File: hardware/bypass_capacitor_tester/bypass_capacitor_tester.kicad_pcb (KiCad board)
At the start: 2 copper layers, 17 x 28.8 mm, 13 parts, among them J1 Coax, J2 Coax, J3 Coax, J4 Conn_01x02, Q1 MMBT2369AL

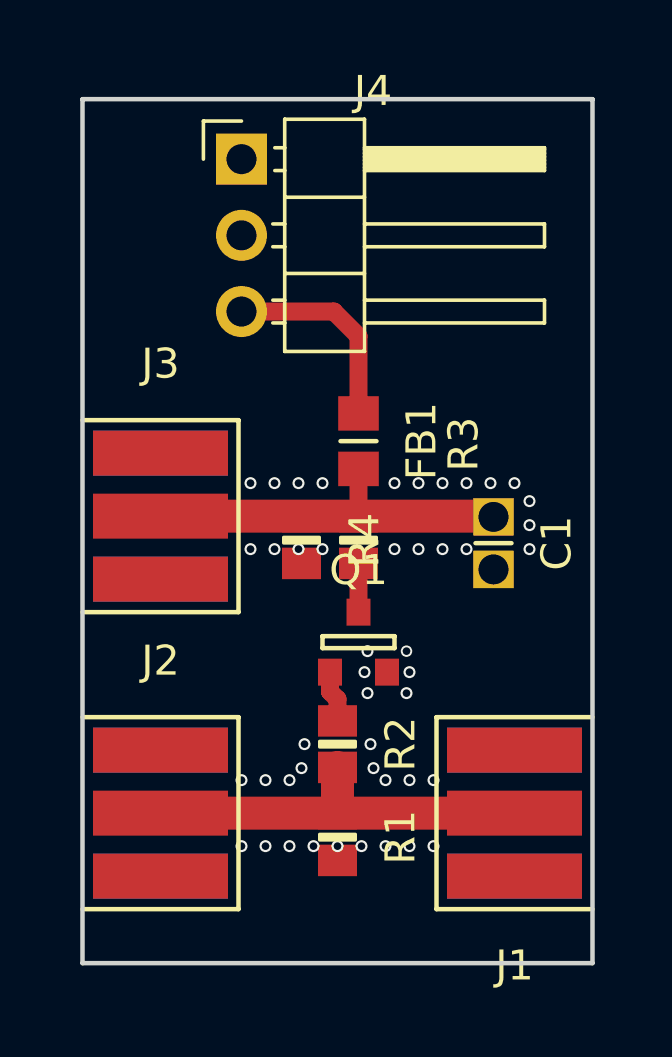
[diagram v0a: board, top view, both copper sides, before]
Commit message: silk placement completed
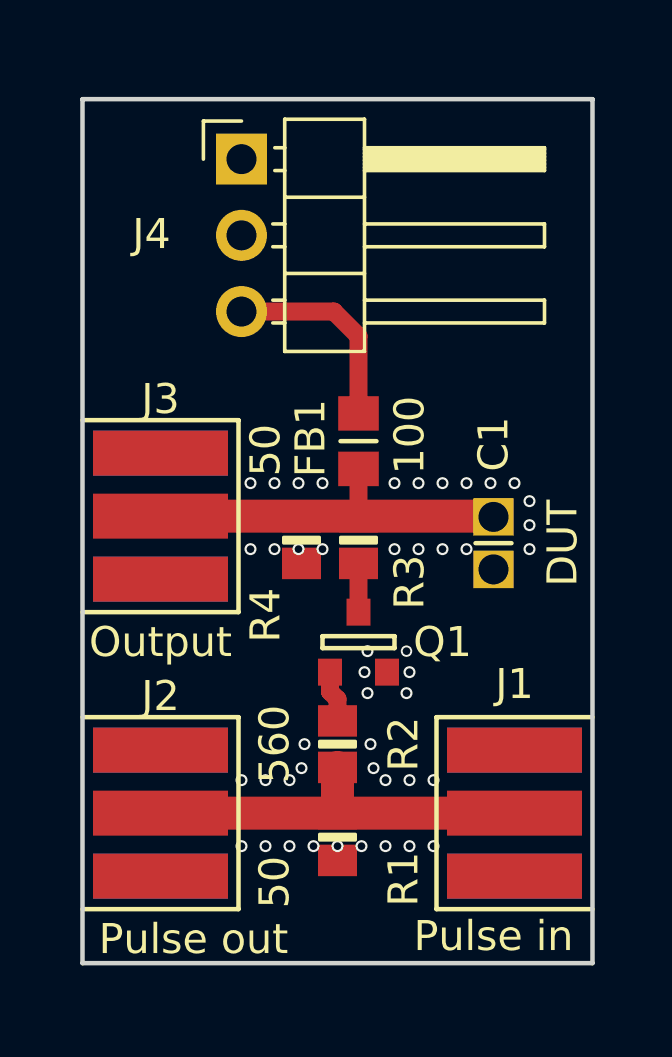
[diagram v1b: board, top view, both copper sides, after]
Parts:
- J1: value Coax -> Pulse in
- J2: value Coax -> Pulse out
- J3: value Coax -> Output
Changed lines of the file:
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@@
     (tags "capacitor 0805 0603 0402 Through hole mixed")
     (attr smd)
-    (fp_text reference C1 (at 0 -2.1 90) (layer F.SilkS)
-      (effects (font (size 1 1) (thickness 0.15)))
-    )
-    (fp_text value DUT (at 0 2.1 90) (layer F.Fab)
+    (fp_text reference C1 (at -3.3 0 90) (layer F.SilkS)
+      (effects (font (size 1 1) (thickness 0.15)))
+    )
+    (fp_text value DUT (at 0 -2.3 90) (layer F.SilkS)
       (effects (font (size 1 1) (thickness 0.15)))
     )
@@
     (descr "Through hole angled pin header, 1x03, 2.54mm pitch, 6mm pin length, single row")
     (tags "Through hole angled pin header THT 1x03 2.54mm single row")
-    (fp_text reference J4 (at 4.385 -2.27) (layer F.SilkS)
+    (fp_text reference J4 (at -3 2.5) (layer F.SilkS)
       (effects (font (size 1 1) (thickness 0.15)))
     )
@@
   (module SquantorConnectors:SMA_edge_6mm2 (layer F.Cu)
     (at 181.1 82.1)
-    (fp_text reference J3 (at 0 -5.08 180) (layer F.SilkS)
-      (effects (font (size 1 1) (thickness 0.15)))
-    )
-    (fp_text value Coax (at 0 4.445 180) (layer F.Fab)
+    (fp_text reference J3 (at 0 -3.9 180) (layer F.SilkS)
+      (effects (font (size 1 1) (thickness 0.15)))
+    )
+    (fp_text value Output (at 0 4.2 180) (layer F.SilkS)
       (effects (font (size 1 1) (thickness 0.15)))
     )
@@
   (module SquantorConnectors:SMA_edge_6mm2 (layer F.Cu)
     (at 181.1 92)
-    (fp_text reference J2 (at 0 -5.08 180) (layer F.SilkS)
-      (effects (font (size 1 1) (thickness 0.15)))
-    )
-    (fp_text value Coax (at 0 4.445 180) (layer F.Fab)
+    (fp_text reference J2 (at 0 -3.9 180) (layer F.SilkS)
+      (effects (font (size 1 1) (thickness 0.15)))
+    )
+    (fp_text value "Pulse out" (at 1.1 4.2 180) (layer F.SilkS)
       (effects (font (size 1 1) (thickness 0.15)))
     )
@@
   (module SquantorConnectors:SMA_edge_6mm2 (layer F.Cu)
     (at 192.9 92 180)
-    (fp_text reference J1 (at 0 -5.08 180) (layer F.SilkS)
-      (effects (font (size 1 1) (thickness 0.15)))
-    )
-    (fp_text value Coax (at 0 4.445 180) (layer F.Fab)
+    (fp_text reference J1 (at 0 4.3 180) (layer F.SilkS)
+      (effects (font (size 1 1) (thickness 0.15)))
+    )
+    (fp_text value "Pulse in" (at 0.7 -4.1 180) (layer F.SilkS)
       (effects (font (size 1 1) (thickness 0.15)))
     )
@@
     (tags "resistor 0805")
     (attr smd)
-    (fp_text reference R4 (at 0 -2.1 90) (layer F.SilkS)
-      (effects (font (size 1 1) (thickness 0.15)))
-    )
-    (fp_text value 50 (at 0 2.1 90) (layer F.Fab)
+    (fp_text reference R4 (at 2.5 1.2 90) (layer F.SilkS)
+      (effects (font (size 1 1) (thickness 0.15)))
+    )
+    (fp_text value 50 (at -3 1.2 90) (layer F.SilkS)
       (effects (font (size 1 1) (thickness 0.15)))
     )
@@
     (tags "resistor 0805")
     (attr smd)
-    (fp_text reference R3 (at -3.2 -3.5 90) (layer F.SilkS)
-      (effects (font (size 1 1) (thickness 0.15)))
-    )
-    (fp_text value 100 (at 0 2.1 90) (layer F.Fab)
+    (fp_text reference R3 (at 1.4 -1.7 90) (layer F.SilkS)
+      (effects (font (size 1 1) (thickness 0.15)))
+    )
+    (fp_text value 100 (at -3.5 -1.7 90) (layer F.SilkS)
       (effects (font (size 1 1) (thickness 0.15)))
     )
@@
     (tags "resistor 0805")
     (attr smd)
-    (fp_text reference R2 (at 0 -2.1 90) (layer F.SilkS)
-      (effects (font (size 1 1) (thickness 0.15)))
-    )
-    (fp_text value 560 (at 0 2.1 90) (layer F.Fab)
+    (fp_text reference R2 (at 0 -2.2 90) (layer F.SilkS)
+      (effects (font (size 1 1) (thickness 0.15)))
+    )
+    (fp_text value 560 (at 0 2.1 90) (layer F.SilkS)
       (effects (font (size 1 1) (thickness 0.15)))
     )
@@
     (tags "resistor 0805")
     (attr smd)
-    (fp_text reference R1 (at 0 -2.1 90) (layer F.SilkS)
-      (effects (font (size 1 1) (thickness 0.15)))
-    )
-    (fp_text value 50 (at 0 2.1 90) (layer F.Fab)
+    (fp_text reference R1 (at 1.4 -2.2 90) (layer F.SilkS)
+      (effects (font (size 1 1) (thickness 0.15)))
+    )
+    (fp_text value 50 (at 1.5 2.1 90) (layer F.SilkS)
       (effects (font (size 1 1) (thickness 0.15)))
     )
@@
   (module SquantorIC:SOT23-3 (layer F.Cu)
     (at 187.7 86.3)
-    (fp_text reference Q1 (at 0 -2.4) (layer F.SilkS)
+    (fp_text reference Q1 (at 2.8 0) (layer F.SilkS)
       (effects (font (size 1 1) (thickness 0.15)))
     )
@@
     (tags "capacitor 0805 0603 mixed")
     (attr smd)
-    (fp_text reference FB1 (at 0 -2.1 90) (layer F.SilkS)
-      (effects (font (size 1 1) (thickness 0.15)))
-    )
-    (fp_text value Ferrite_Bead (at 0 2.1 90) (layer F.Fab)
-      (effects (font (size 1 1) (thickness 0.15)))
-    )
+    (fp_text reference FB1 (at -0.1 1.6 90) (layer F.SilkS)
+      (effects (font (size 1 1) (thickness 0.15)))
+    )
+    (fp_text value Ferrite_Bead (at -0.6 -4.1 90) (layer F.Fab) hide
+      (effects (font (size 1 1) (thickness 0.15)))
+    )
